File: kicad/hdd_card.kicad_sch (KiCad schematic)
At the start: 23 parts, among them J1 POISK, J2 ICSP, J3 SDCARD, J4 UART, U1 28C256, U2 74LS245, U3 28C256, U4 PIC18F47Q10-xP, U5 74LS00, U6 74LS32, U7 74LS74, U8 74LS05

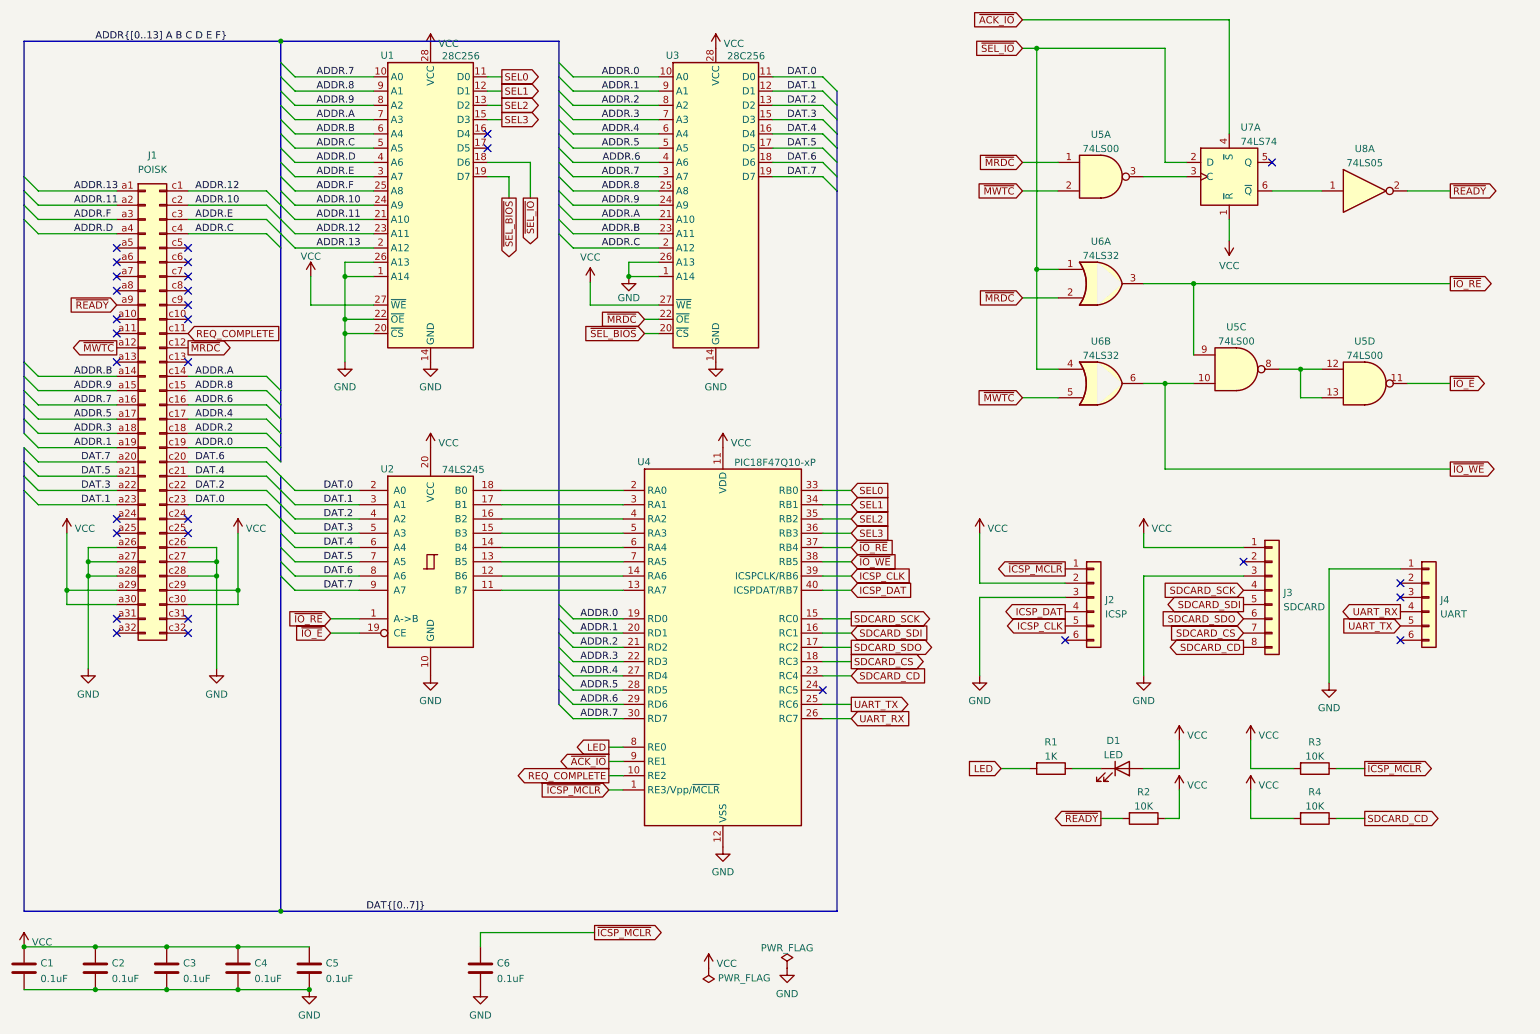
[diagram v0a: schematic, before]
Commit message: SEL4
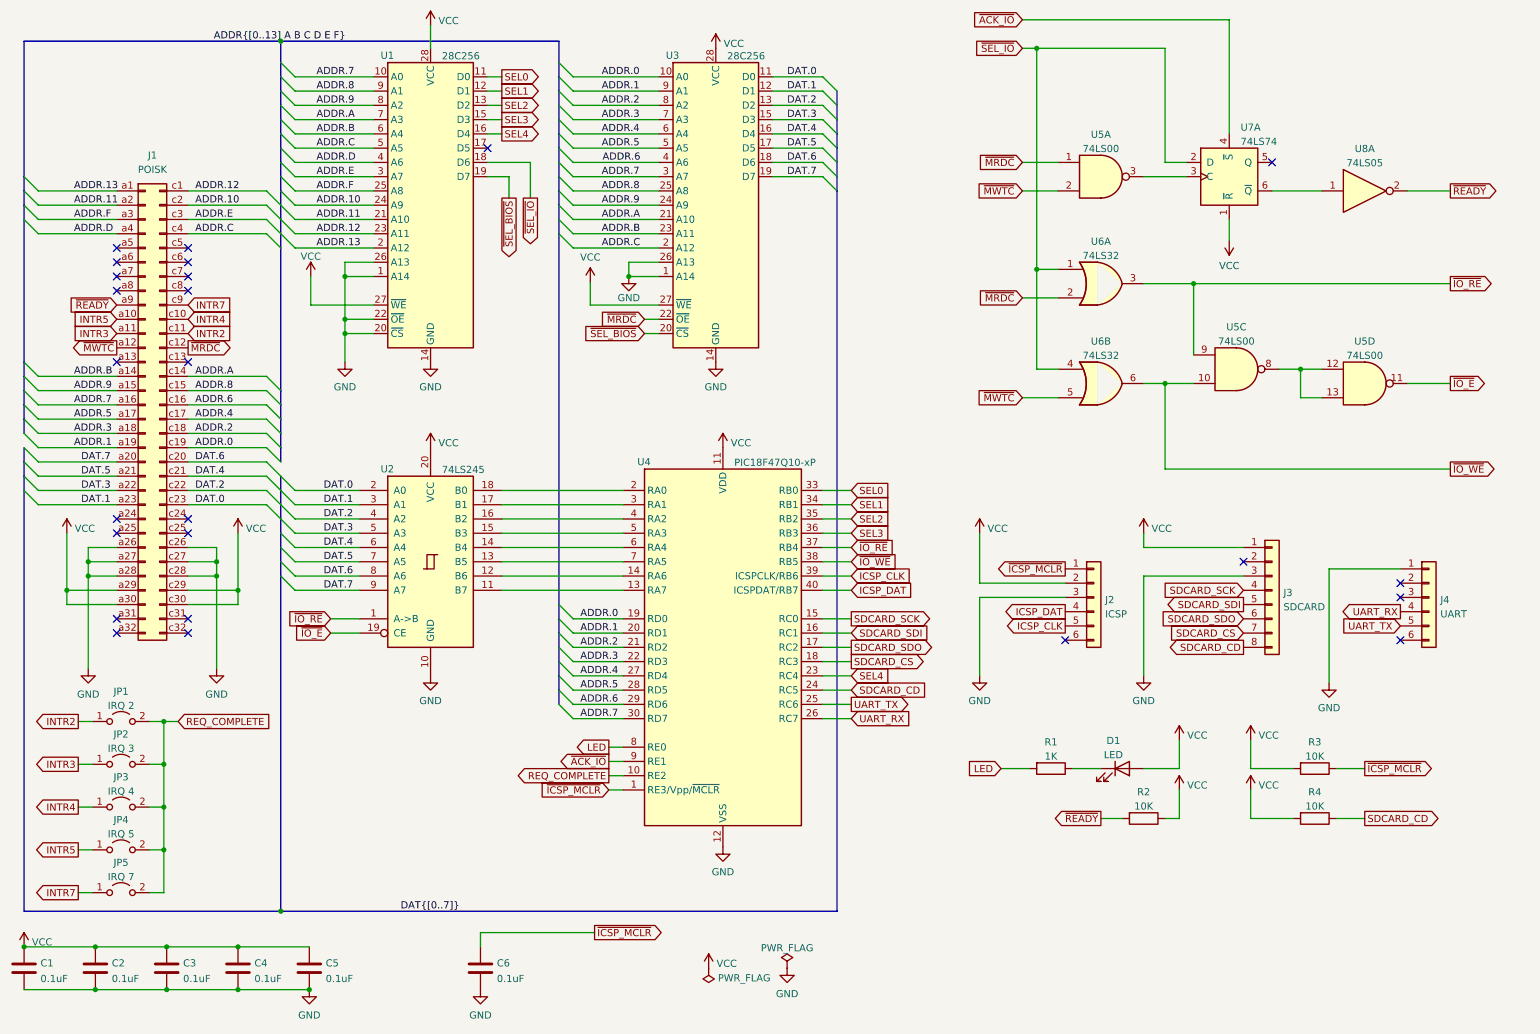
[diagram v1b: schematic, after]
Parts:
- added JP1: IRQ 2, Connector_PinHeader_2.54mm:PinHeader_1x02_P2.54mm_Vertical, symbol Jumper:Jumper_2_Open
- added JP2: IRQ 3, Connector_PinHeader_2.54mm:PinHeader_1x02_P2.54mm_Vertical, symbol Jumper:Jumper_2_Open
- added JP3: IRQ 4, Connector_PinHeader_2.54mm:PinHeader_1x02_P2.54mm_Vertical, symbol Jumper:Jumper_2_Open
- added JP4: IRQ 5, Connector_PinHeader_2.54mm:PinHeader_1x02_P2.54mm_Vertical, symbol Jumper:Jumper_2_Open
- added JP5: IRQ 7, Connector_PinHeader_2.54mm:PinHeader_1x02_P2.54mm_Vertical, symbol Jumper:Jumper_2_Open
- D1: footprint (none) -> LED_THT:LED_D5.0mm
- J2, J4: footprint (none) -> Connector_PinHeader_2.54mm:PinHeader_1x06_P2.54mm_Vertical
- J3: footprint (none) -> Connector_PinHeader_2.54mm:PinHeader_1x08_P2.54mm_Vertical
- R1, R2, R3, R4: footprint (none) -> Resistor_THT:R_Axial_DIN0207_L6.3mm_D2.5mm_P7.62mm_Horizontal
- U1, U3: footprint (none) -> Package_DIP:DIP-28_W15.24mm
- U2: footprint (none) -> Package_DIP:DIP-20_W7.62mm
- U5, U6, U7, U8: footprint (none) -> Package_DIP:DIP-14_W7.62mm
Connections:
- net REQ_COMPLETE: now also JP1.2 (B), JP2.2 (B), JP3.2 (B), JP4.2 (B), JP5.2 (B); no longer J1.c11 (Pin_c11)
- net SDCARD_CD: now also U4.24 (RC5); no longer U4.23 (RC4)
- net SEL4: now reaches U1.16 (D4)
- net SEL4: now also U4.23 (RC4)
- net INTR5: now reaches J1.a10 (Pin_a10)
- net INTR5: now also JP4.1 (A)
- net INTR3: now reaches J1.a11 (Pin_a11)
- net INTR3: now also JP2.1 (A)
- net INTR4: now reaches J1.c10 (Pin_c10)
- net INTR4: now also JP3.1 (A)
- net INTR7: now reaches J1.c9 (Pin_c9)
- net INTR7: now also JP5.1 (A)
- new net INTR2: J1.c11 (Pin_c11), JP1.1 (A)
- no-connect marks 31 -> 25

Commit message: WIP
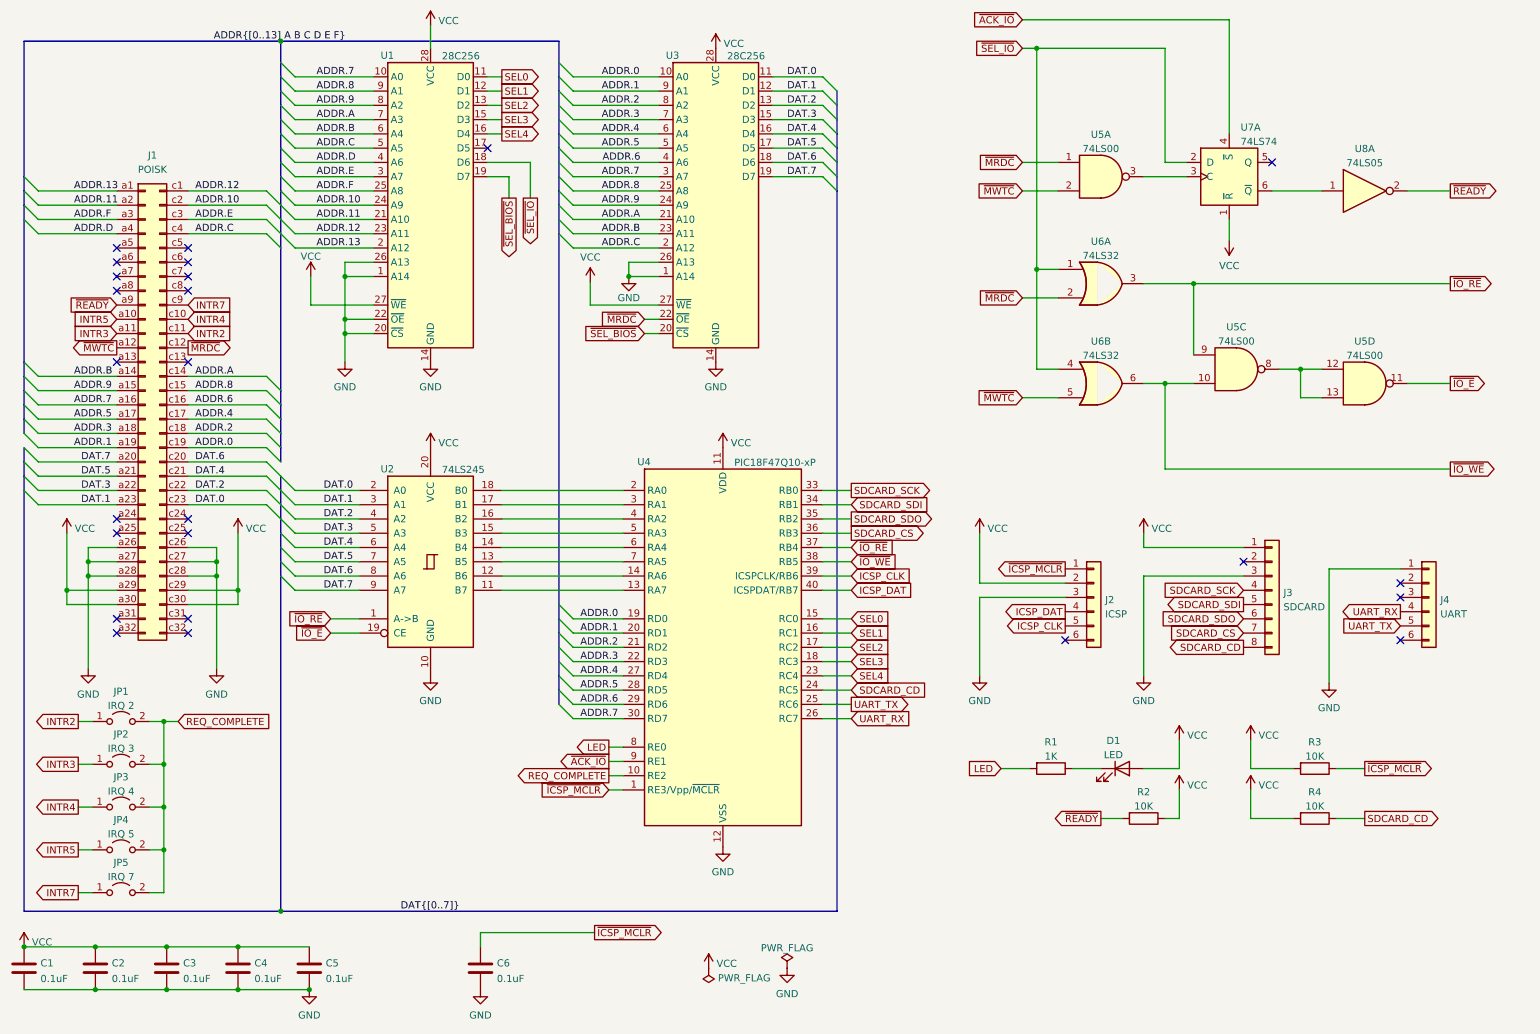
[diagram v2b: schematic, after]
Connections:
- net SDCARD_CS: now also U4.36 (RB3); no longer U4.18 (RC3)
- net SDCARD_SCK: now also U4.33 (RB0); no longer U4.15 (RC0)
- net SDCARD_SDI: now also U4.34 (RB1); no longer U4.16 (RC1)
- net SDCARD_SDO: now also U4.35 (RB2); no longer U4.17 (RC2)
- net SEL0: now also U4.15 (RC0); no longer U4.33 (RB0)
- net SEL1: now also U4.16 (RC1); no longer U4.34 (RB1)
- net SEL2: now also U4.17 (RC2); no longer U4.35 (RB2)
- net SEL3: now also U4.18 (RC3); no longer U4.36 (RB3)
